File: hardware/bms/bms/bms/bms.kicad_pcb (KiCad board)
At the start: 2 copper layers, 17.5 x 43.2 mm, 24 parts, among them J1 OUTPUT, J2 INPUT_CELL, J3 INPUT_LOGIC, J4 Conn_01x02_Pin, Q1 Q_NPN_BEC

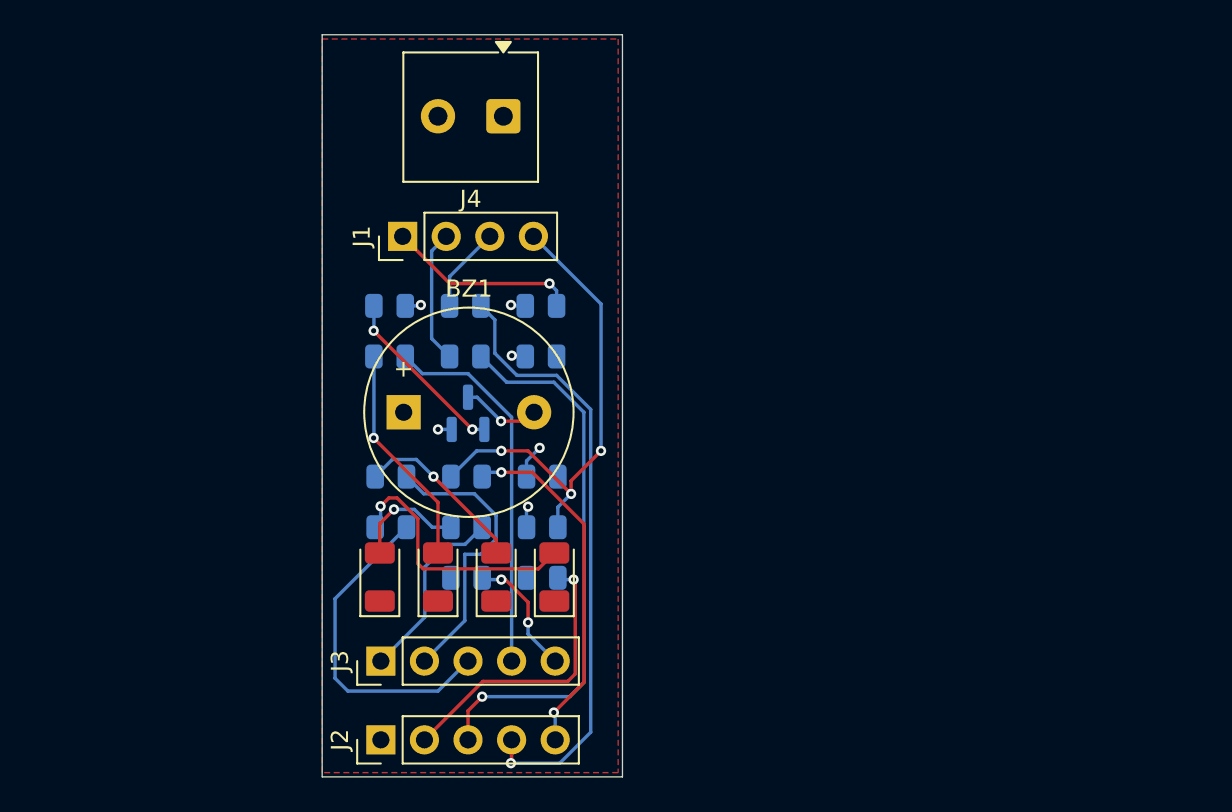
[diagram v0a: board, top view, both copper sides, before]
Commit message: New commit
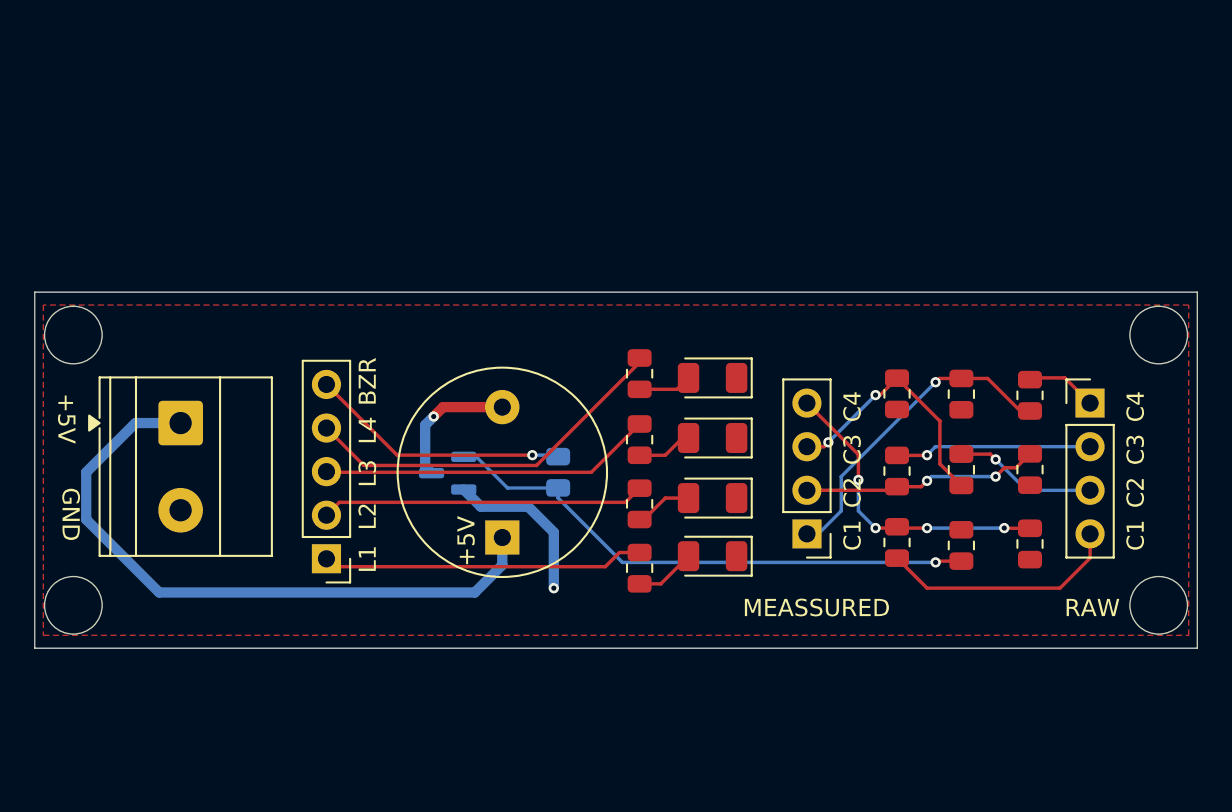
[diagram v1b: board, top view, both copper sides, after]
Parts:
- removed J2: INPUT_CELL, Connector_PinHeader_2.54mm:PinHeader_1x05_P2.54mm_Vertical
- added J5: Screw_Terminal_01x02, TerminalBlock_Phoenix:TerminalBlock_Phoenix_MKDS-1,5-2-5.08_1x02_P5.08mm_Horizontal, F.Cu at (137.0, 90.6)
- J4: value Conn_01x02_Pin -> INPUT_CELL1; footprint TerminalBlock_Phoenix:TerminalBlock_Phoenix_MKDS-1-2-3.81_1x02_P3.81mm_Horizontal -> Connector_PinHeader_2.54mm:PinHeader_1x04_P2.54mm_Vertical
- RBOTT5, RBOTT6, RBOTT7, RBOTT8, RTOP11, RTOP12, RTOP13, RTOP14, RTOP5, RTOP6, RTOP7, RTOP8, RTOP9: moved to F.Cu
- moved J4 38.1 mm to (190.0, 89.5), turned to 0 degrees
- moved RTOP11 36.1 mm to (182.5, 97.8), turned to -90 degrees
- moved RTOP6 30.4 mm to (182.5, 93.4), turned to -90 degrees
- moved RTOP5 30.4 mm to (186.5, 89.0), turned to -90 degrees
- moved J1 29.3 mm to (173.5, 97.1), turned to 180 degrees
- moved RBOTT8 28.4 mm to (186.5, 97.7), turned to -90 degrees
- moved RBOTT7 28.4 mm to (186.5, 93.3), turned to -90 degrees
- moved RTOP7 26.0 mm to (178.8, 93.4), turned to -90 degrees
- moved RTOP8 25.4 mm to (178.8, 97.6), turned to 90 degrees
- moved RBOTT5 25.0 mm to (182.5, 88.9), turned to -90 degrees
- moved RBOTT6 20.9 mm to (178.8, 88.9), turned to -90 degrees
- moved D2 19.8 mm to (168.0, 88.0), turned to 180 degrees
- moved D1 19.4 mm to (168.0, 98.4), turned to 180 degrees
- moved RTOP14 15.4 mm to (163.8, 91.6), turned to -90 degrees
- moved RTOP12 14.6 mm to (163.8, 87.8), turned to -90 degrees
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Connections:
- J4 pad 1: unconnected-(J4-Pin_1-Pad1) -> RAW_CELL1
- J4 pad 2: unconnected-(J4-Pin_2-Pad2) -> RAW_CELL2
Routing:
- net /5V: track 0.00 -> 38.5 mm
- net RAW_CELL3: track 35.6 -> 8.37 mm
- net Net-(Q1-B): track 10.3 -> 31.9 mm, vias 2 -> 1
- net RAW_CELL2: track 32.2 -> 11.5 mm
- net RAW_CELL1: track 16.9 -> 4.15 mm, vias 1 -> 0
- net Net-(D4-A): track 15.3 -> 3.27 mm, vias 1 -> 0
- net /MEASS_CELL4: track 28.3 -> 18.0 mm, vias 3 -> 4
- net Net-(D2-A): track 13.0 -> 3.12 mm, vias 1 -> 0
- net /MEASS_CELL3: track 5.02 -> 14.7 mm, vias 0 -> 2
- net /LED1: track 10.8 -> 18.8 mm
- net /BUZZER_GATE: track 7.34 -> 15.2 mm, vias 2 -> 1
- net /MEASS_CELL1: track 11.2 -> 18.7 mm
- net Net-(D3-A): track 10.2 -> 3.37 mm, vias 1 -> 0
- net RAW_CELL4: track 20.6 -> 14.1 mm, vias 2 -> 0
- net /MEASS_CELL2: track 7.78 -> 13.9 mm, vias 0 -> 2
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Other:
- board size 17.5 x 43.2 mm -> 67.8 x 20.8 mm
- board text added: "+5V"
- board text added: "BZR"
- board text added: "C1"
- board text added: "C2"
- board text added: "C3"
- board text added: "C4"
- board text added: "GND"
- board text added: "L1"
- board text added: "L2"
- board text added: "L3"
- board text added: "L4"
- board text added: "MEASSURED"
- board text added: "Made by: Javier E Veras Seda"
- board text added: "RAW"
